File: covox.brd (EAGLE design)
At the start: 80 x 50 mm, 24 parts, among them CN1 POWERJACK, IC1 74HCT373N

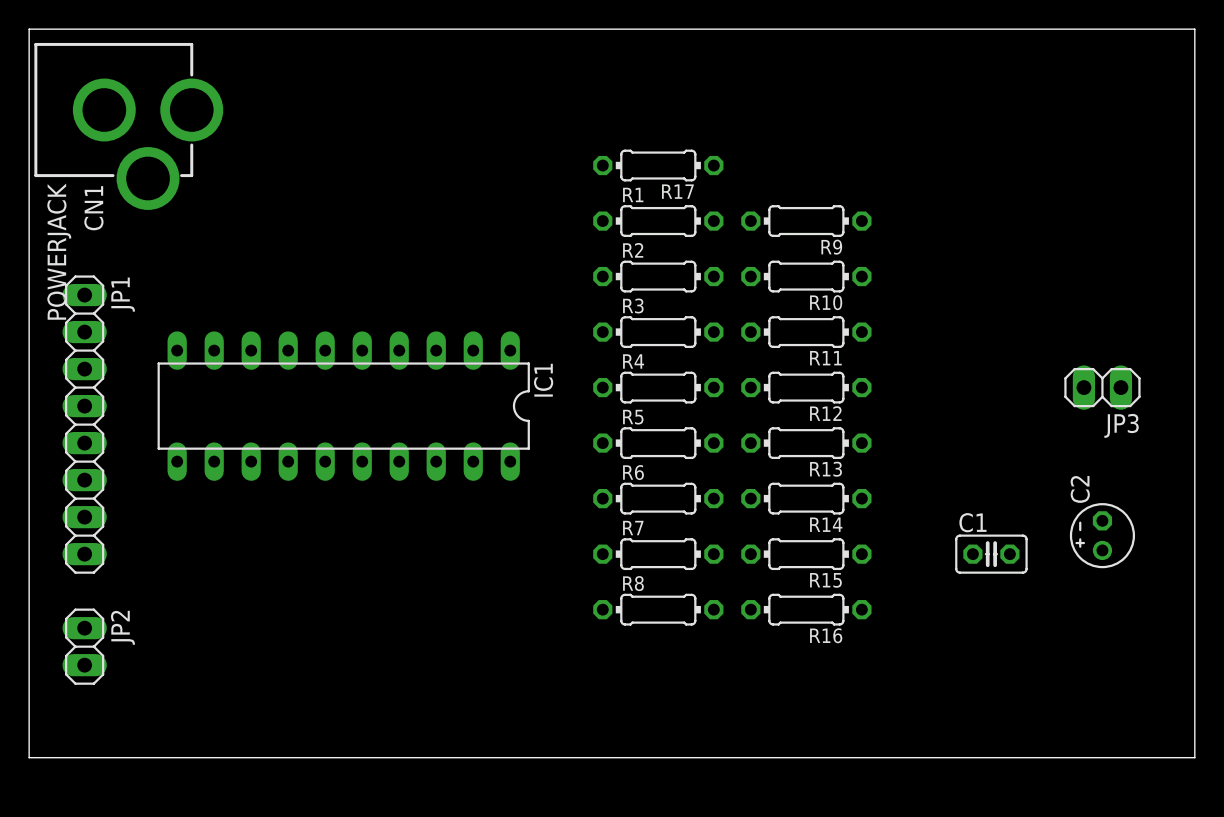
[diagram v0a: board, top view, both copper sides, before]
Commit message: updates
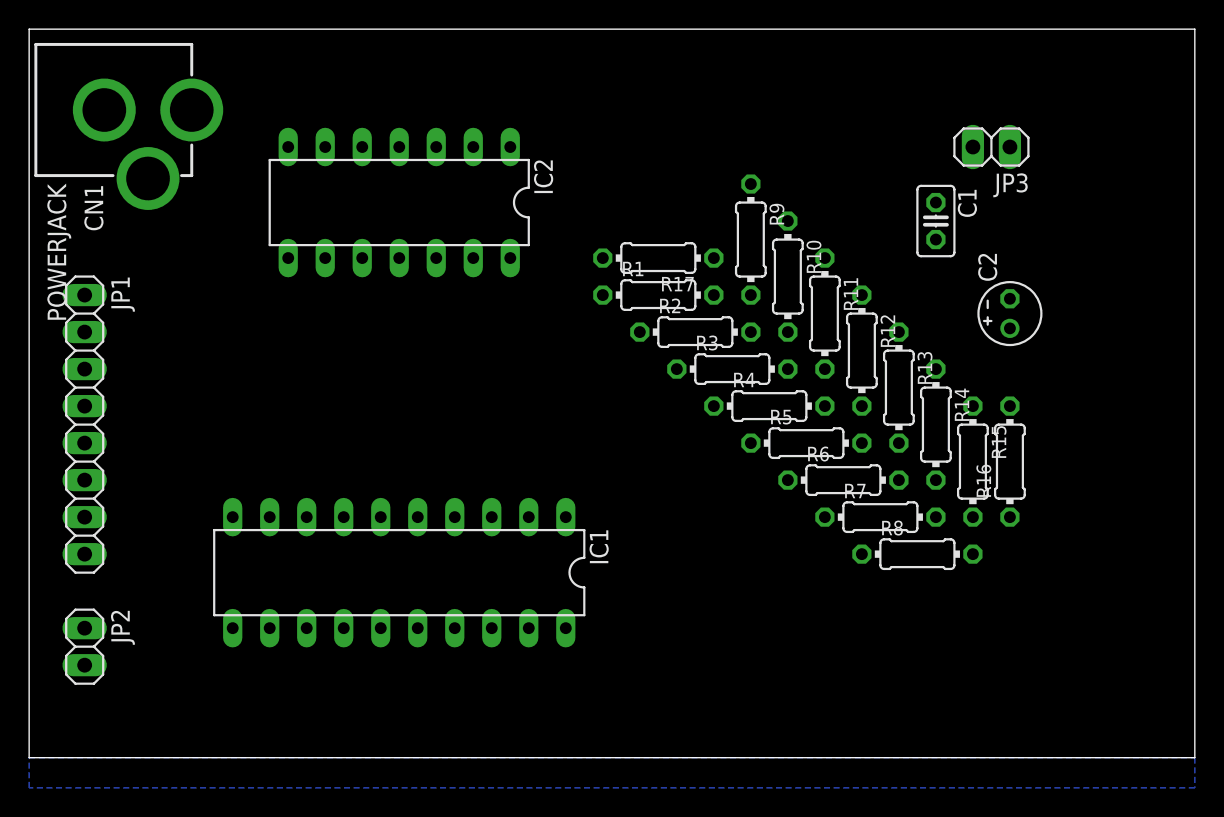
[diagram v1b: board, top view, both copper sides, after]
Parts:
- added IC2: 74HC164N, 74xx-eu:DIL14
- C1: value 10uF -> 0.01uF
- C2: value (none) -> 0.1uF
- R10, R11, R12, R13, R14, R15, R16, R9: value 7.5k -> 7k5
- moved C1 23.2 mm to (62.2, 36.8), turned to 270 degrees
- moved R8 18.2 mm to (61.0, 14.0)
- moved JP3 18.2 mm to (66.0, 41.9)
- moved R16 17.3 mm to (67.3, 20.3), turned to 90 degrees
- moved C2 16.5 mm to (67.3, 30.5)
- moved R7 15.5 mm to (58.4, 16.5)
- moved R15 13.1 mm to (64.8, 20.3), turned to 270 degrees
- moved R6 12.8 mm to (55.9, 19.1)
- moved IC1 12.0 mm to (25.4, 12.7)
- moved R14 10.2 mm to (62.2, 22.9), turned to 270 degrees
- moved R5 10.2 mm to (53.3, 21.6)
- moved R4 7.73 mm to (50.8, 24.1)
- moved R13 7.41 mm to (59.7, 25.4), turned to 270 degrees
- moved R17 6.35 mm to (43.2, 34.3)
- moved R3 5.68 mm to (48.3, 26.7)
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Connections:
- removed net N$16: C1.2, C2.+, R16.2
- new net AOUT: C1.1, C2.+, R16.2
- net GND: now also C1.2, IC2.7; no longer C1.1
- net N$18: now also IC2.3
- net N$19: now also IC2.4
- net N$20: now also IC2.5
- net N$21: now also IC2.6
- net N$22: now also IC2.10
- net N$23: now also IC2.11
- net N$24: now also IC2.12
- net N$25: now also IC2.13
- net VCC: now also IC2.14
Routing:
- added copper zone on layer 16, net GND
